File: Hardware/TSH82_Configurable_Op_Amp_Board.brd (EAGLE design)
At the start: 160 x 100 mm, 33 parts, among them U1 TSH82

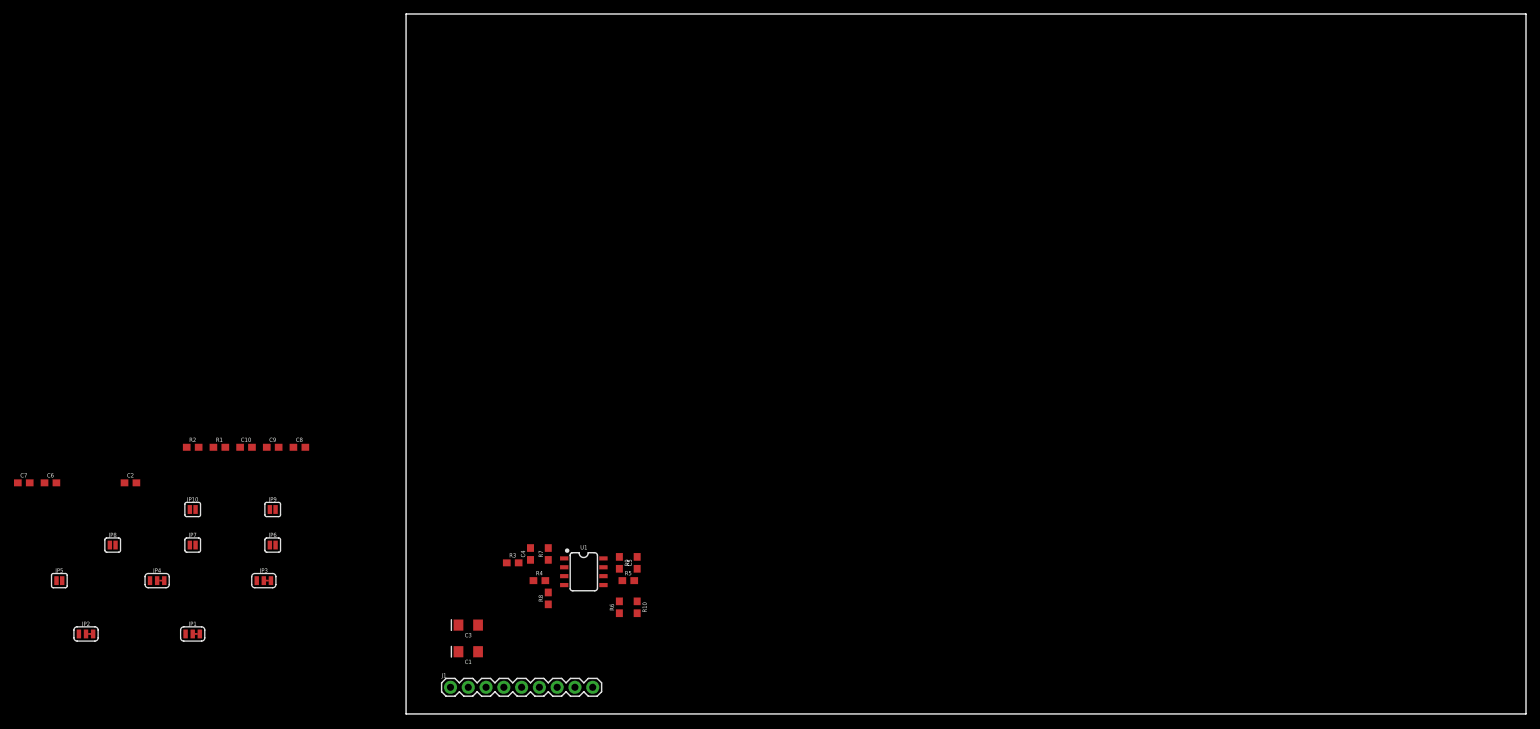
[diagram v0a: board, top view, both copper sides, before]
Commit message: Close to done, labels, layout, etc.
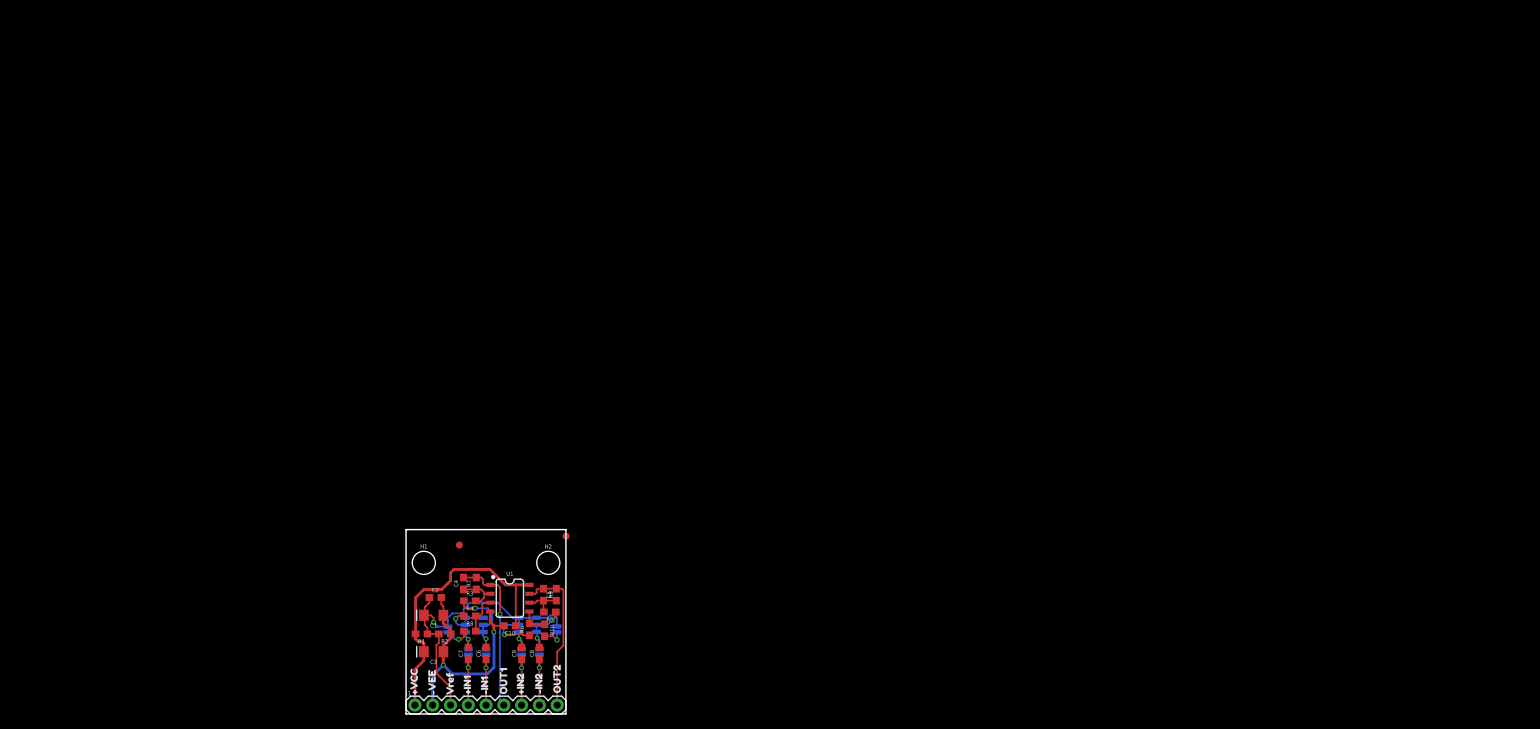
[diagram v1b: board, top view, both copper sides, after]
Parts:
- added FD1, FD2: FIDUCIAL1X2, SparkFun-Aesthetics:FIDUCIAL-1X2
- added H1, H2: STAND-OFF, SparkFun-Hardware:STAND-OFF
- added LOGO1: SFE_LOGO_NAME_FLAME.2_INCH, SparkFun-Aesthetics:SFE_LOGO_NAME_FLAME_.2
- added U$1: (no value), buzzard_labels:VREF9
- added U$2: (no value), buzzard_labels:#VEE2
- added U$3: (no value), buzzard_labels:#VCC1
- added U$4: (no value), buzzard_labels:#IN13
- added U$5: (no value), buzzard_labels:#IN14
- added U$6: (no value), buzzard_labels:OUT15
- added U$7: (no value), buzzard_labels:#IN26
- added U$8: (no value), buzzard_labels:#IN27
- added U$9: (no value), buzzard_labels:OUT28
- moved FRAME1 72.0 mm to (-8.89, -10.2)
- moved C7 68.0 mm to (8.89, 8.64), turned to 90 degrees
- moved C6 66.8 mm to (11.4, 8.64), turned to 90 degrees
- moved JP5 61.8 mm to (11.4, 8.89), flipped to the bottom, turned to 270 degrees
- moved JP8 60.4 mm to (16.5, 8.89), flipped to the bottom, turned to 270 degrees
- moved JP10 54.8 mm to (21.6, 12.1), flipped to the bottom, turned to 90 degrees
- moved JP2 54.2 mm to (8.48, 12.7), flipped to the bottom, turned to 90 degrees
- moved JP4 52.0 mm to (16.1, 12.7), flipped to the bottom, turned to 90 degrees
- moved JP7 51.8 mm to (19.1, 8.89), flipped to the bottom, turned to 270 degrees
- moved C2 46.5 mm to (4.19, 16.6)
- moved C9 46.2 mm to (16.5, 8.64), turned to 90 degrees
- moved C10 45.5 mm to (14.8, 12.6), turned to 180 degrees
- moved C8 45.2 mm to (19.1, 8.64), turned to 90 degrees
- moved R2 44.8 mm to (5.54, 11.4), turned to 180 degrees
- moved JP1 41.5 mm to (11.0, 12.7), flipped to the bottom, turned to 270 degrees
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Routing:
- net VREF: track 0.00 -> 47.1 mm, vias 0 -> 1
- net VCC: track 0.00 -> 42.0 mm
- net VNEG: track 0.00 -> 34.8 mm, vias 0 -> 2
- net OUT1: track 0.00 -> 23.2 mm, vias 0 -> 1
- net OUT2: track 0.00 -> 22.3 mm
- net -IN2: track 0.00 -> 8.40 mm, vias 0 -> 1
- net -IN1: track 0.00 -> 8.40 mm, vias 0 -> 1
- net +IN2: track 0.00 -> 8.40 mm, vias 0 -> 1
- net +IN1: track 0.00 -> 8.40 mm, vias 0 -> 1
- net N$4: track 0.00 -> 7.93 mm, vias 0 -> 1
- net N$16: track 0.00 -> 6.93 mm, vias 0 -> 1
- net N$1: track 0.00 -> 6.13 mm
- net N$2: track 0.00 -> 5.76 mm
- net N$11: track 0.00 -> 5.62 mm
- net N$9: track 0.00 -> 4.18 mm, vias 0 -> 1
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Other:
- board size 160 x 100 mm -> 22.8 x 26.3 mm

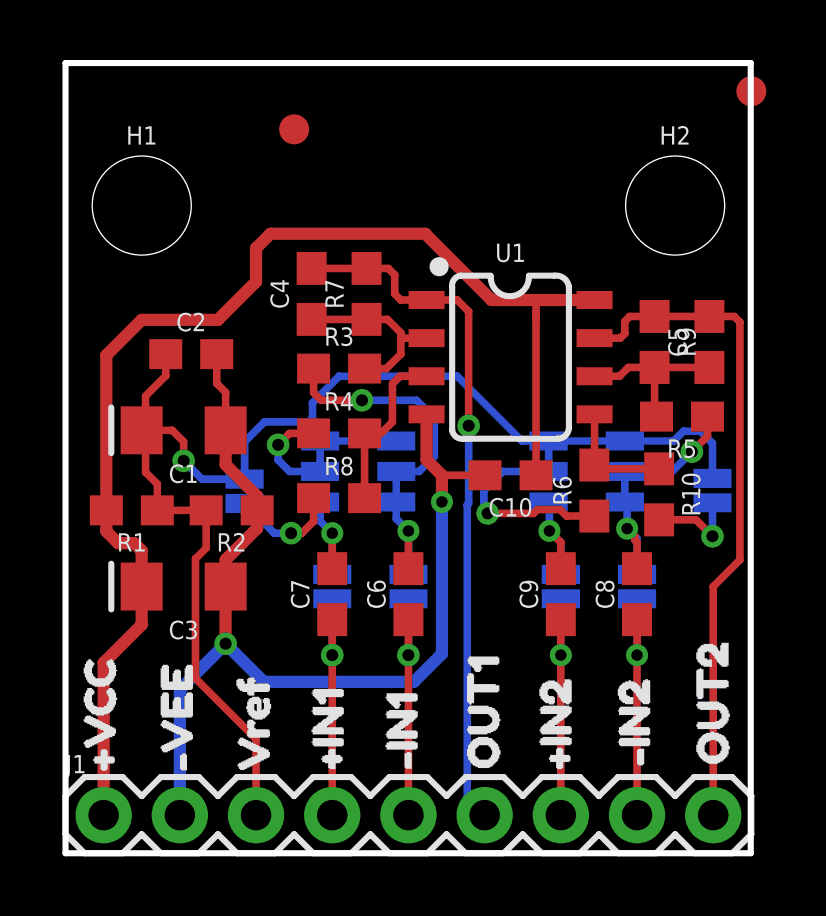
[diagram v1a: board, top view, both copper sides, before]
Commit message: Ready for review.
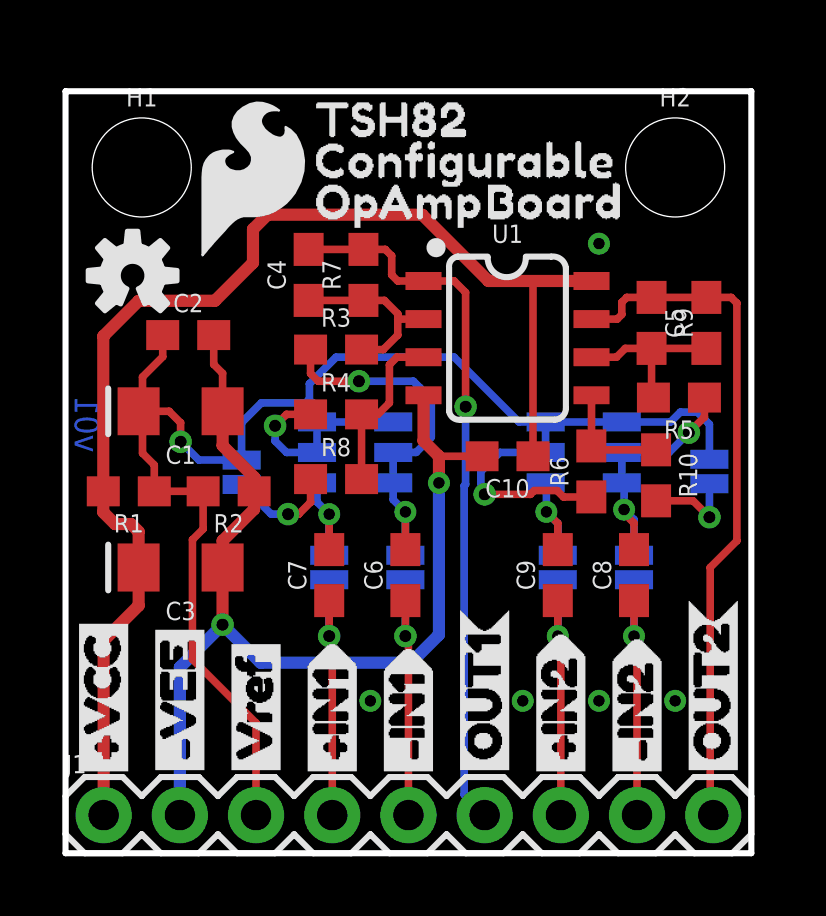
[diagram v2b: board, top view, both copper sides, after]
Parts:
- removed FD1, FD2: FIDUCIAL1X2, SparkFun-Aesthetics:FIDUCIAL-1X2
- added LOGO2: SFE_LOGO_NAME_FLAME.1_INCH, SparkFun-Aesthetics:SFE_LOGO_NAME_FLAME_.1
- added LOGO3: OSHW-LOGOS, SparkFun-Aesthetics:OSHW-LOGO-S
- added U$10, U$11: (no value), buzzard_labels (5):OUT17
- added U$12, U$13: (no value), buzzard_labels (5):#IN24
- added U$14, U$16: (no value), buzzard_labels (5):#IN25
- added U$15, U$17: (no value), buzzard_labels (5):OUT28
- added U$22, U$26: (no value), buzzard_labels (4):TSH820
- added U$23, U$27: (no value), buzzard_labels (4):CONFIGURABLE1
- added U$24, U$28: (no value), buzzard_labels (4):OPAMP2
- added U$25, U$29: (no value), buzzard_labels (4):BOARD3
- added U$30: (no value), buzzard_labels (5):#VCC0
- LOGO1: value SFE_LOGO_NAME_FLAME.2_INCH -> SFE_LOGO_FLAME.2_INCH; device SparkFun-Aesthetics:SFE_LOGO_NAME_FLAME_.2 -> SparkFun-Aesthetics:SFE_LOGO_FLAME_.2
- U$1: device buzzard_labels:VREF9 -> buzzard_labels (5):#VEE1
- U$2: device buzzard_labels:#VEE2 -> buzzard_labels (5):#VEE1
- U$3: device buzzard_labels:#VCC1 -> buzzard_labels (5):#VCC0
- U$4: device buzzard_labels:#IN13 -> buzzard_labels (5):VREF6
- U$5: device buzzard_labels:#IN14 -> buzzard_labels (5):VREF6
- U$6: device buzzard_labels:OUT15 -> buzzard_labels (5):#IN12
- U$7: device buzzard_labels:#IN26 -> buzzard_labels (5):#IN12
- U$8: device buzzard_labels:#IN27 -> buzzard_labels (5):#IN13
- U$9: device buzzard_labels:OUT28 -> buzzard_labels (5):#IN13
- moved LOGO1 21.5 mm to (4.22, 19.7), flipped to the top
- moved U$9 10.1 mm to (11.4, 2.21), flipped to the bottom
- moved U$8 7.52 mm to (11.4, 2.21)
- moved U$7 7.45 mm to (8.89, 2.21)
- moved U$6 5.04 mm to (8.89, 2.21), flipped to the bottom
- moved U$5 4.86 mm to (6.35, 2.21), flipped to the bottom
- moved U$1 2.49 mm to (3.81, 2.21)
- moved U$4 2.41 mm to (6.35, 2.21)
- moved H1 1.27 mm to (2.54, 22.9)
- moved H2 1.27 mm to (20.3, 22.9)
- moved C5 0.64 mm to (21.4, 17.7)
- moved C7 0.64 mm to (8.79, 9.27)
- moved C8 0.64 mm to (18.9, 9.27)
- moved C9 0.64 mm to (16.4, 9.27)
- moved R3 0.64 mm to (9.02, 16.8)
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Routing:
- net VREF: track 47.1 -> 47.8 mm
- net OUT2: track 22.3 -> 22.9 mm
- net -IN2: track 8.40 -> 9.07 mm
- net -IN1: track 8.40 -> 9.07 mm
- net +IN2: track 8.40 -> 9.07 mm
- net +IN1: track 8.40 -> 9.07 mm
- net OUT1: track 23.2 -> 23.9 mm
- net VNEG: track 34.8 -> 35.3 mm, vias 2 -> 7
- net VCC: track 42.0 -> 42.6 mm
- added copper zone on layer 1, net VNEG
- added copper zone on layer 16, net VNEG
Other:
- board size 22.8 x 26.3 mm -> 22.9 x 25.4 mm
- board text added: "JP1"
- board text added: "JP10"
- board text added: "JP2"
- board text added: "JP3"
- board text added: "JP4"
- board text added: "JP5"
- board text added: "JP6"
- board text added: "JP7"
- board text added: "JP8"
- board text added: "JP9"
- board text added: "Pete Dokter"
- board text added: "v01"
